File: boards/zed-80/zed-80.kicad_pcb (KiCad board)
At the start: 2 copper layers, 107.5 x 72.5 mm, 33 parts, among them J401 TYPE-C-31-M-12, SW201 SW_Push, U201 GD74LS04, U202 Z84C0010PEC, U301 TT74LS32BI, U302 AT28C256-15PU, U303 HM628128BLP-10, U401 CH340C, U402 MC68B50P, Y201 7.3728 MHz

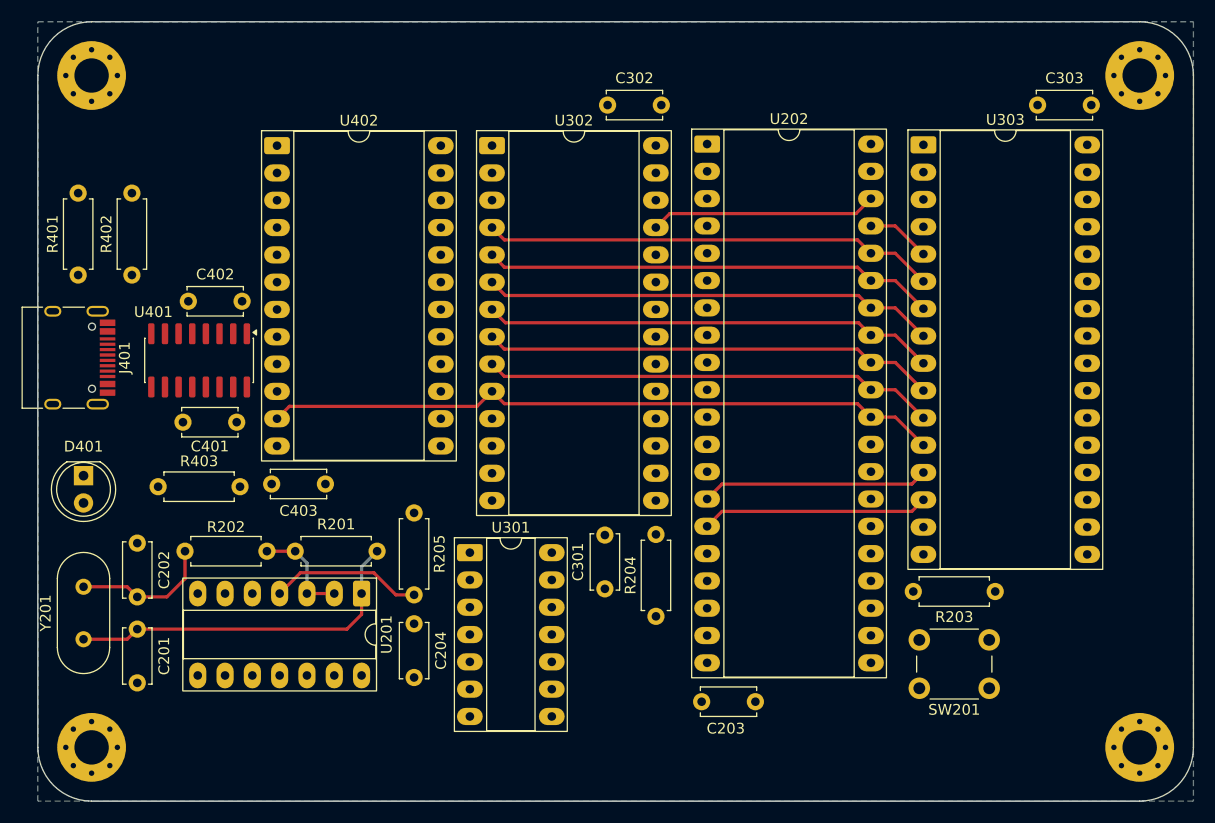
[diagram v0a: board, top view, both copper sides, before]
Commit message: Initial PCB design for main board
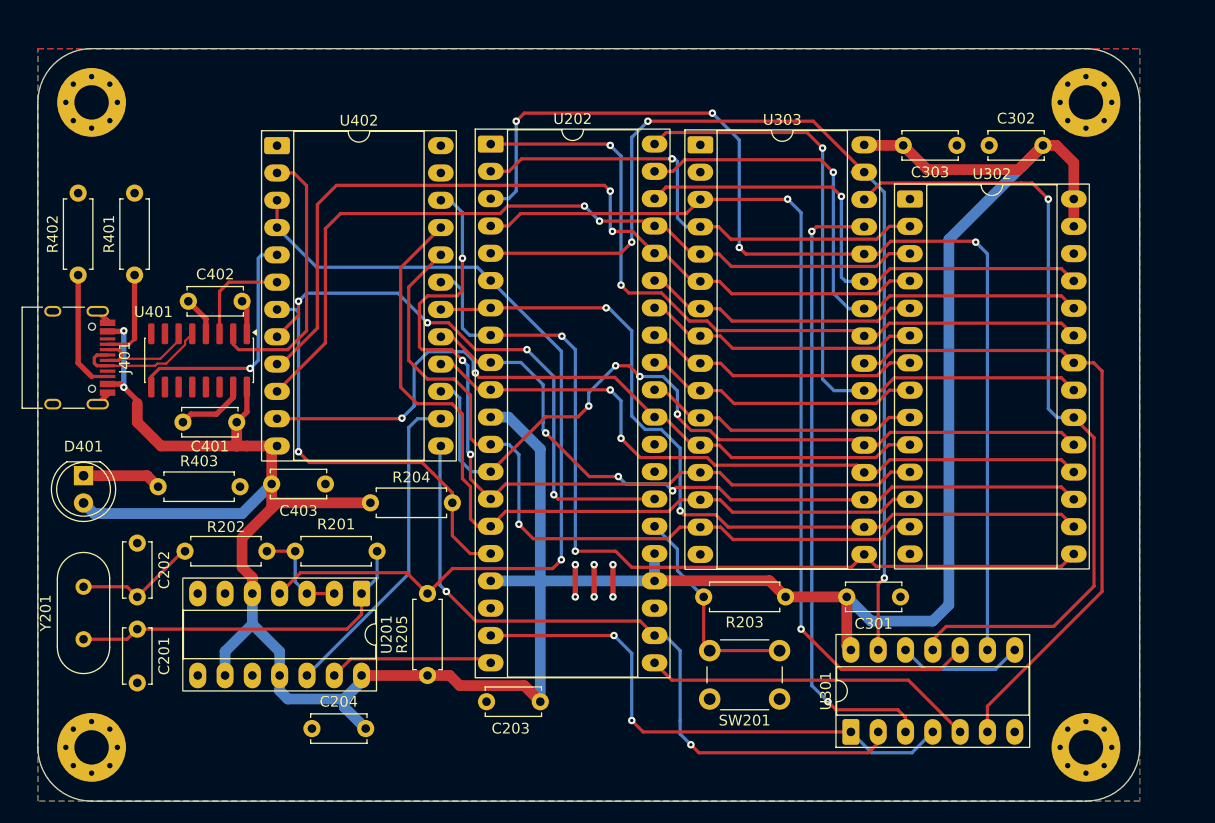
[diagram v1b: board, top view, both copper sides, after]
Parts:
- moved U302 39.2 mm to (161.1, 56.5)
- moved U301 39.2 mm to (155.6, 106.1), turned to 90 degrees
- moved C302 35.7 mm to (168.5, 51.5)
- moved R204 28.6 mm to (110.9, 84.8), turned to 0 degrees
- moved C301 27.5 mm to (160.2, 93.5), turned to 180 degrees
- moved U303 20.8 mm to (141.6, 51.5)
- moved U202 20.1 mm to (122.1, 51.4)
- moved C203 20.0 mm to (121.7, 103.2)
- moved SW201 19.5 mm to (142.5, 98.5)
- moved R203 19.5 mm to (149.6, 93.5)
- moved R205 15.2 mm to (116.2, 100.8), turned to 90 degrees
- moved C204 13.6 mm to (105.5, 105.8), turned to 0 degrees
- moved C303 8.39 mm to (165.5, 51.5), turned to 180 degrees
- moved MH102 5.59 mm to (177.5, 47.5)
- moved R401 5.25 mm to (89.0, 63.6)
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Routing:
- net VBUS: track 0.00 -> 278.4 mm, vias 0 -> 2
- net /CPU/A13: track 0.00 -> 102.4 mm, vias 0 -> 4
- net /CPU/A15: track 0.00 -> 94.1 mm, vias 0 -> 3
- net /CPU/A14: track 0.00 -> 86.3 mm, vias 0 -> 2
- net /CPU/D3: track 0.00 -> 84.3 mm, vias 0 -> 2
- net /CPU/D4: track 0.00 -> 76.4 mm, vias 0 -> 2
- net /CPU/D7: track 0.00 -> 75.6 mm, vias 0 -> 4
- net /Memory/~{ROM}: track 0.00 -> 75.1 mm, vias 0 -> 1
- net /CPU/D2: track 0.00 -> 72.1 mm, vias 0 -> 1
- net /CPU/A11: track 0.00 -> 69.6 mm, vias 0 -> 2
- net /CPU/A7: track 5.96 -> 75.1 mm, vias 0 -> 2
- net /CPU/D5: track 0.00 -> 68.9 mm, vias 0 -> 3
- net /CPU/CLK: track 14.2 -> 82.6 mm, vias 0 -> 1
- net /CPU/~{WR}: track 0.00 -> 66.6 mm, vias 0 -> 2
- net /CPU/D6: track 0.00 -> 66.1 mm, vias 0 -> 2
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- added copper zone on F.Cu, net GND
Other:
- board size 107.5 x 72.5 mm -> 102.5 x 70 mm
